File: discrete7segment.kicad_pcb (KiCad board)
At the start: 2 copper layers, 111.8 x 94 mm, 76 parts, among them P1 CONN_01X02, Q1 Q_NPN_BEC, Q2 Q_NPN_BEC, Q3 Q_NPN_BEC, Q4 Q_NPN_BEC, Q5 Q_NPN_BEC, Q6 Q_NPN_BEC, Q7 Q_NPN_BEC, U1 555, U2 4017

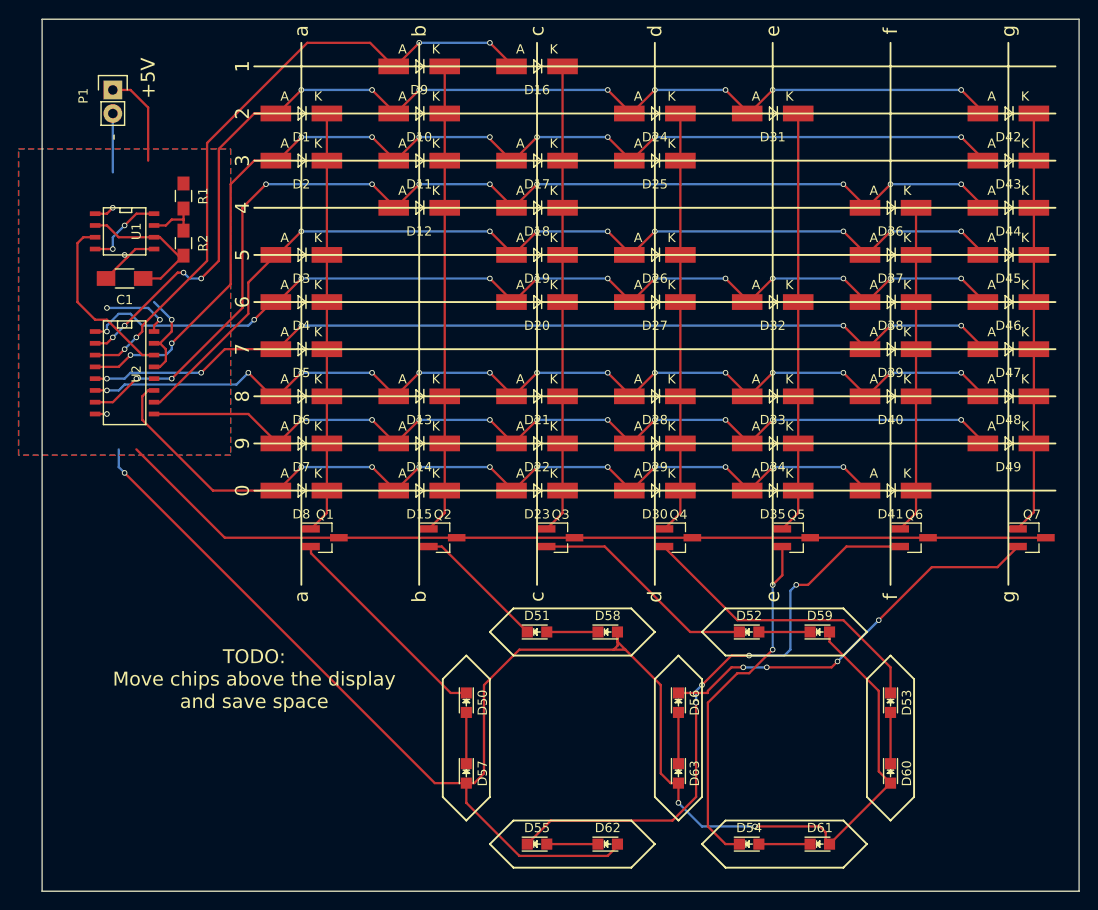
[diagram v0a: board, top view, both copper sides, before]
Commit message: layout from scratch
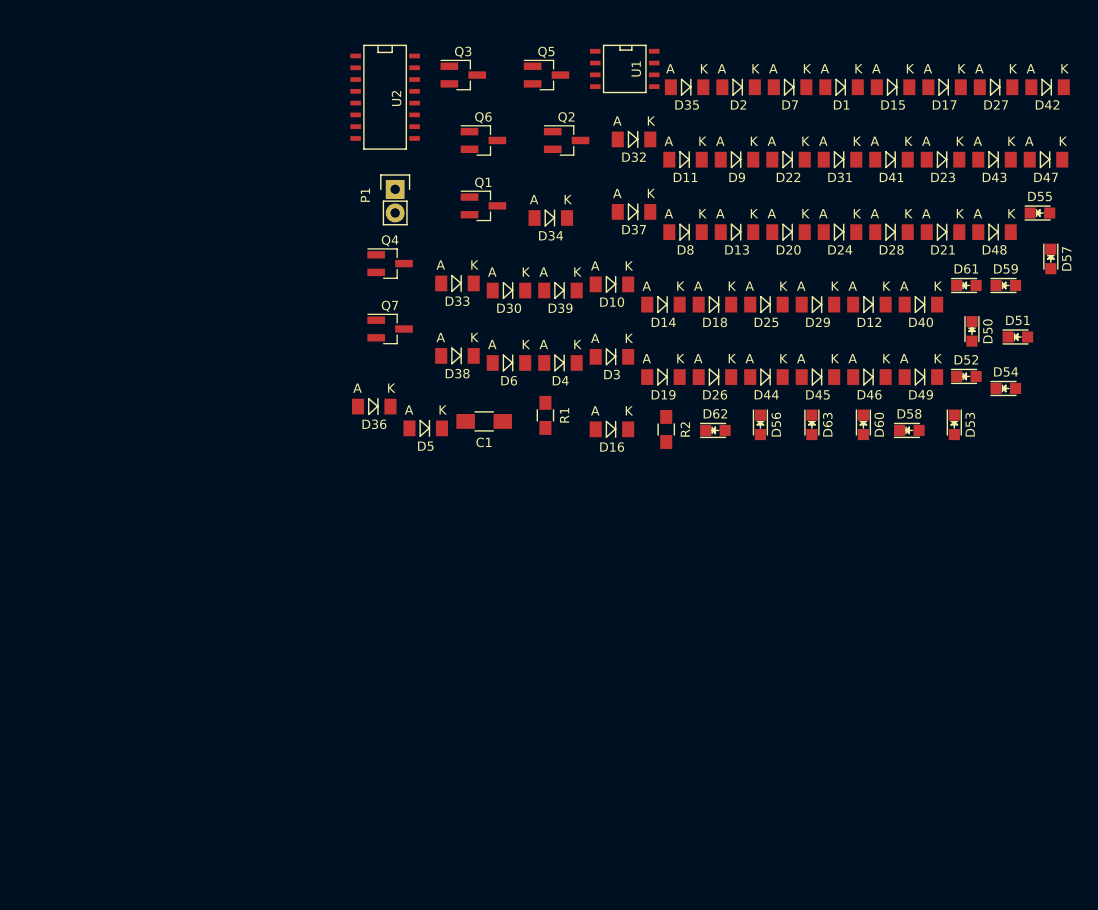
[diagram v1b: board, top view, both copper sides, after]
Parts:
- D1, D10, D11, D12, D13, D14, D15, D16, D17, D18, D19, D2, D20, D21, D22, D23, D24, D25, D26, D27, D28, D29, D3, D30, D31, D32, D33, D34, D35, D36, D37, D38, D39, D4, D40, D41, D42, D43, D44, D45, D46, D47, D48, D49, D5, D6, D7, D8, D9: footprint Diodes_SMD:MiniMELF_Handsoldering -> Diodes_SMD:MiniMELF_Standard
- moved D55 87.0 mm to (178.7, 84.4)
- moved D57 83.9 mm to (179.8, 89.3)
- moved Q7 72.7 mm to (108.6, 96.9)
- moved D50 67.6 mm to (171.3, 97.1)
- moved D15 67.1 mm to (162.8, 70.8)
- moved D7 65.2 mm to (151.7, 70.8)
- moved Q6 63.1 mm to (118.7, 76.6)
- moved D61 62.2 mm to (170.7, 92.2)
- moved D51 60.8 mm to (176.3, 97.7)
- moved D36 59.6 mm to (106.9, 105.2)
- moved D1 58.3 mm to (157.3, 70.8)
- moved U1 56.7 mm to (133.9, 68.9)
- moved Q5 56.7 mm to (125.5, 69.5)
- moved D23 56.4 mm to (168.2, 78.6)
- moved D54 56.4 mm to (175.0, 103.3)
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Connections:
- D16 pad 1: /c -> /b
- D17 pad 2: Net-(D11-Pad2) -> Net-(D17-Pad2)
- D18 pad 2: Net-(D12-Pad2) -> Net-(D11-Pad2)
- D19 pad 2: Net-(D19-Pad2) -> Net-(D12-Pad2)
- D21 pad 2: Net-(D13-Pad2) -> Net-(D21-Pad2)
- D22 pad 2: Net-(D14-Pad2) -> Net-(D13-Pad2)
- D23 pad 2: Net-(D15-Pad2) -> Net-(D14-Pad2)
- D24 pad 1: /d -> /c
- D24 pad 2: Net-(D1-Pad2) -> Net-(D15-Pad2)
- D25 pad 1: /d -> /c
- D25 pad 2: Net-(D11-Pad2) -> Net-(D16-Pad2)
- D26 pad 2: Net-(D19-Pad2) -> Net-(D1-Pad2)
- D27 pad 2: Net-(D20-Pad2) -> Net-(D11-Pad2)
- D28 pad 2: Net-(D13-Pad2) -> Net-(D20-Pad2)
- D29 pad 2: Net-(D14-Pad2) -> Net-(D21-Pad2)
- D3 pad 2: Net-(D19-Pad2) -> Net-(D20-Pad2)
- D30 pad 2: Net-(D15-Pad2) -> Net-(D14-Pad2)
- D31 pad 1: /e -> /d
- D31 pad 2: Net-(D1-Pad2) -> Net-(D15-Pad2)
- D32 pad 1: /e -> /d
- D32 pad 2: Net-(D20-Pad2) -> Net-(D16-Pad2)
- D33 pad 2: Net-(D13-Pad2) -> Net-(D1-Pad2)
- D34 pad 2: Net-(D14-Pad2) -> Net-(D21-Pad2)
- D35 pad 2: Net-(D15-Pad2) -> Net-(D14-Pad2)
- D36 pad 1: /f -> /e
- D36 pad 2: Net-(D12-Pad2) -> Net-(D16-Pad2)
- D37 pad 2: Net-(D19-Pad2) -> Net-(D12-Pad2)
- D39 pad 2: Net-(D39-Pad2) -> Net-(D21-Pad2)
- D4 pad 2: Net-(D20-Pad2) -> Net-(D21-Pad2)
- D40 pad 2: Net-(D13-Pad2) -> Net-(D14-Pad2)
- D42 pad 1: /g -> /f
- D42 pad 2: Net-(D1-Pad2) -> Net-(D16-Pad2)
- D43 pad 2: Net-(D11-Pad2) -> Net-(D1-Pad2)
- D44 pad 2: Net-(D12-Pad2) -> Net-(D11-Pad2)
- D45 pad 2: Net-(D19-Pad2) -> Net-(D12-Pad2)
- D47 pad 2: Net-(D39-Pad2) -> Net-(D21-Pad2)
- D48 pad 2: Net-(D13-Pad2) -> Net-(D14-Pad2)
- D49 pad 2: Net-(D14-Pad2) -> Net-(D15-Pad2)
- D5 pad 2: Net-(D39-Pad2) -> Net-(D13-Pad2)
- D6 pad 2: Net-(D13-Pad2) -> Net-(D14-Pad2)
- D7 pad 2: Net-(D14-Pad2) -> Net-(D15-Pad2)
- D8 pad 2: Net-(D15-Pad2) -> Net-(D16-Pad2)
- D9 pad 2: Net-(D16-Pad2) -> Net-(D17-Pad2)
- U2 pad 1: Net-(D20-Pad2) -> Net-(D21-Pad2)
- U2 pad 10: Net-(D19-Pad2) -> Net-(D20-Pad2)
- U2 pad 11: Net-(D15-Pad2) -> Net-(D16-Pad2)
- U2 pad 12: Net-(U2-Pad12) -> (no net)
- U2 pad 3: Net-(D16-Pad2) -> Net-(D17-Pad2)
- U2 pad 5: Net-(D39-Pad2) -> Net-(D13-Pad2)
- U2 pad 6: Net-(D13-Pad2) -> Net-(D14-Pad2)
- U2 pad 9: Net-(D14-Pad2) -> Net-(D15-Pad2)
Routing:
- net GND: track 201.0 -> 0.00 mm, vias 7 -> 0
- net +5V: track 128.7 -> 0.00 mm, vias 4 -> 0
- net Net-(D1-Pad2): track 121.8 -> 0.00 mm, vias 12 -> 0
- net Net-(D11-Pad2): track 120.2 -> 0.00 mm, vias 10 -> 0
- net Net-(D12-Pad2): track 119.2 -> 0.00 mm, vias 10 -> 0
- net Net-(D13-Pad2): track 109.4 -> 0.00 mm, vias 14 -> 0
- net Net-(D20-Pad2): track 108.5 -> 0.00 mm, vias 12 -> 0
- net Net-(D19-Pad2): track 106.4 -> 0.00 mm, vias 8 -> 0
- net Net-(D14-Pad2): track 101.4 -> 0.00 mm, vias 10 -> 0
- net Net-(D39-Pad2): track 101.3 -> 0.00 mm, vias 6 -> 0
- net Net-(D15-Pad2): track 95.8 -> 0.00 mm, vias 10 -> 0
- net Net-(D16-Pad2): track 70.2 -> 0.00 mm, vias 4 -> 0
- net Net-(D55-Pad1): track 63.9 -> 0.00 mm, vias 4 -> 0
- net /c: track 50.6 -> 0.00 mm
- net /b: track 50.6 -> 0.00 mm
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- removed copper zone on F.Cu, net +5V
- removed copper zone on B.Cu, net GND
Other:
- board outline removed
- board text removed: "+5V"
- board text removed: "-"
- board text removed: "0"
- board text removed: "1"
- board text removed: "2"
- board text removed: "3"
- board text removed: "4"
- board text removed: "5"
- board text removed: "6"
- board text removed: "7"
- board text removed: "8"
- board text removed: "9"
- board text removed: "TODO: Move chips above the display and save space"
- board text removed: "a"
- board text removed: "b"
- board text removed: "c"
- board text removed: "d"
- board text removed: "e"
- board text removed: "f"
- board text removed: "g"

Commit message: layout finished
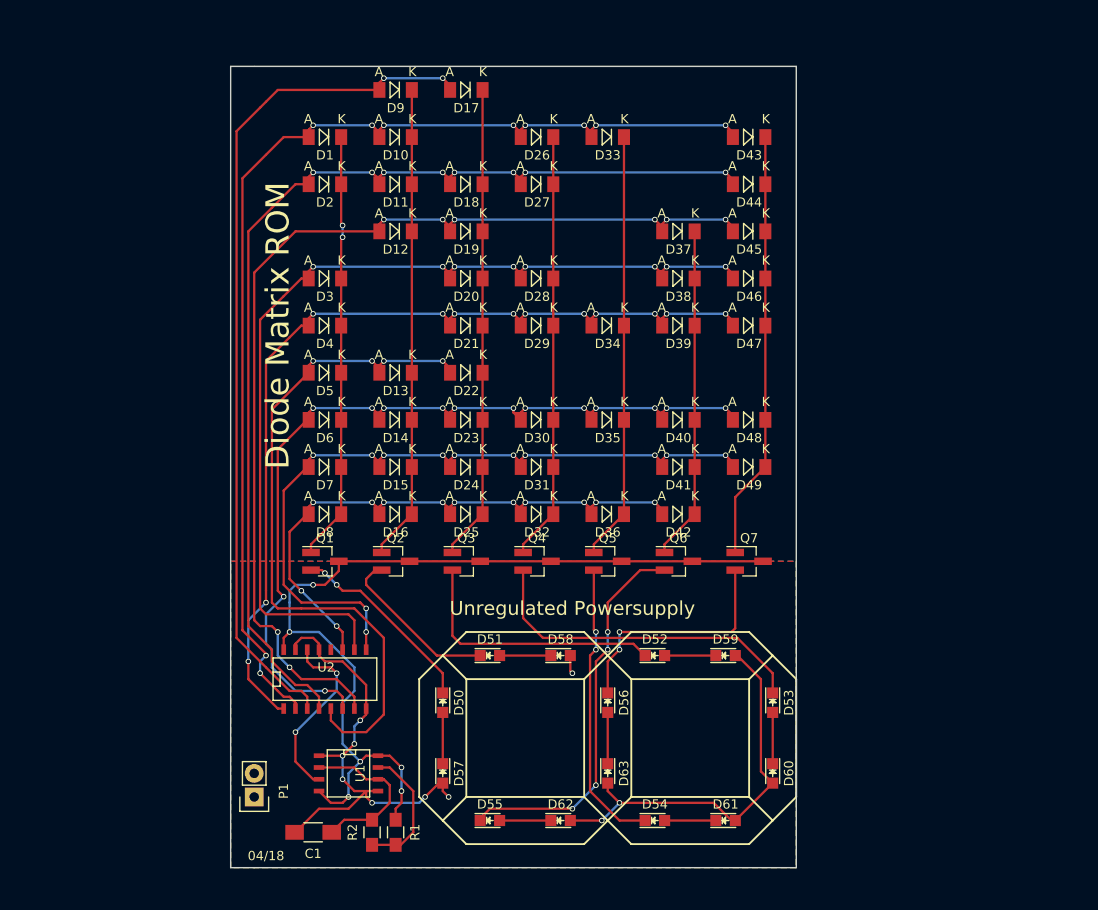
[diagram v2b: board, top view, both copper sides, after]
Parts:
- moved D55 88.3 mm to (119.4, 149.9)
- moved D57 85.8 mm to (114.3, 144.8)
- moved U1 81.6 mm to (104.1, 144.8)
- moved D50 69.7 mm to (114.3, 137.2)
- moved D15 67.5 mm to (109.2, 111.8)
- moved P1 67.2 mm to (94.0, 147.3), turned to 180 degrees
- moved D51 66.5 mm to (119.4, 132.1)
- moved D7 64.7 mm to (101.6, 111.8)
- moved D61 63.2 mm to (144.8, 149.9)
- moved U2 63.1 mm to (101.6, 134.6), turned to 0 degrees
- moved D42 60.8 mm to (139.7, 116.8)
- moved D54 60.0 mm to (137.2, 149.9)
- moved D23 58.5 mm to (116.8, 106.7)
- moved D1 55.9 mm to (101.6, 76.2)
- moved R2 53.8 mm to (106.7, 151.1), turned to 90 degrees
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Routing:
- net Net-(D1-Pad2): track 0.00 -> 119.7 mm, vias 0 -> 10
- net Net-(D11-Pad2): track 0.00 -> 112.7 mm, vias 0 -> 8
- net Net-(D12-Pad2): track 0.00 -> 111.3 mm, vias 0 -> 8
- net Net-(D20-Pad2): track 0.00 -> 100.8 mm, vias 0 -> 8
- net +5V: track 0.00 -> 99.0 mm, vias 0 -> 6
- net Net-(D21-Pad2): track 0.00 -> 97.2 mm, vias 0 -> 12
- net GND: track 0.00 -> 96.1 mm, vias 0 -> 10
- net Net-(D17-Pad2): track 0.00 -> 92.8 mm, vias 0 -> 2
- net Net-(D14-Pad2): track 0.00 -> 90.6 mm, vias 0 -> 14
- net Net-(D15-Pad2): track 0.00 -> 79.2 mm, vias 0 -> 12
- net Net-(D13-Pad2): track 0.00 -> 74.2 mm, vias 0 -> 4
- net Net-(D16-Pad2): track 0.00 -> 59.4 mm, vias 0 -> 12
- net /b: track 0.00 -> 51.2 mm
- net /c: track 0.00 -> 51.2 mm
- net /a: track 0.00 -> 46.5 mm, vias 0 -> 2
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- added copper zone on F.Cu, net +5V
- added copper zone on B.Cu, net GND
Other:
- board outline added: 61 x 86.4 mm
- board text added: "04/18"
- board text added: "Diode Matrix ROM"
- board text added: "Unregulated Powersupply"
